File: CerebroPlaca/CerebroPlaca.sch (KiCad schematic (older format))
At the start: 39 parts

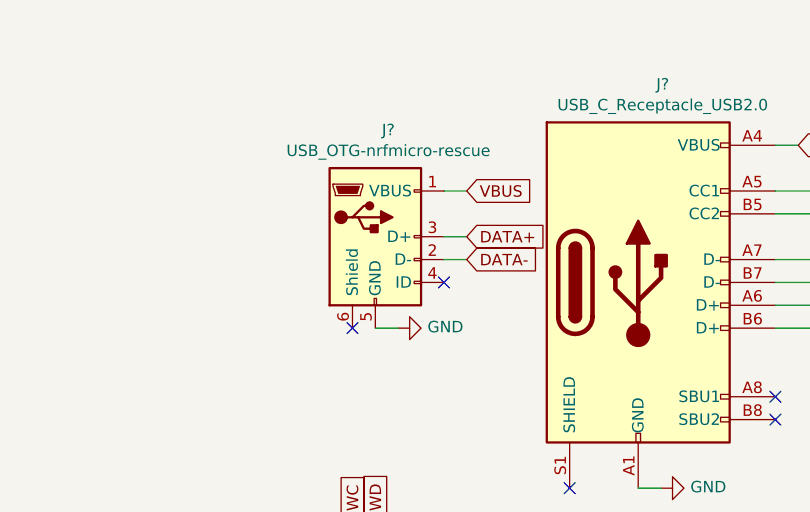
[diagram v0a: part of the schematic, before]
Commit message: se queda con el USB-C
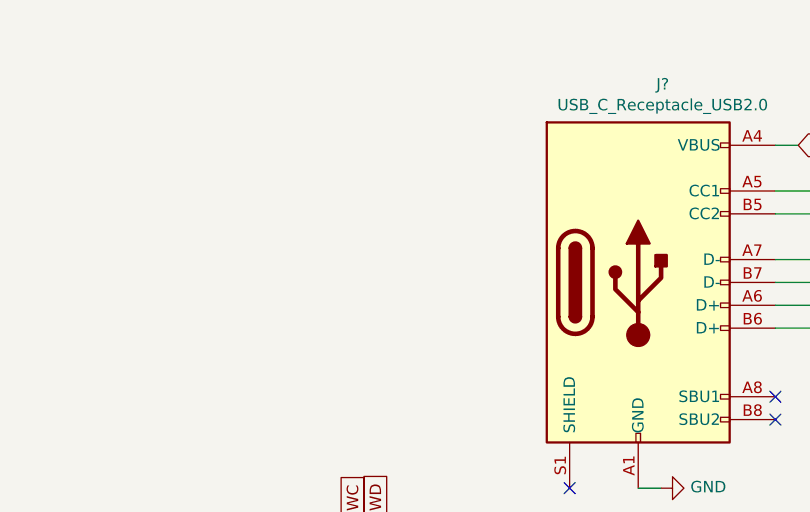
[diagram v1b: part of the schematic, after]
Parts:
- removed J?: USB_OTG-nrfmicro-rescue, symbol cerebro-rescue:USB_OTG-nrfmicro-rescue
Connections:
- no-connect marks 7 -> 5
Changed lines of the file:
@@
 P0.26
-$Comp
-L cerebro-rescue:USB_OTG-nrfmicro-rescue J?
-U 1 1 5E504B1F
-P 5400 1700
-F 0 "J?" H 5457 2167 50  0000 C CNN
-F 1 "USB_OTG-nrfmicro-rescue" H 5457 2076 50  0000 C CNN
-F 2 "" H 5550 1650 50  0001 C CNN
-F 3 "" H 5550 1650 50  0001 C CNN
-	1    5400 1700
-	1    0    0    -1
-$EndComp
 $Comp
 L Connector:USB_C_Receptacle_USB2.0 J?
@@
 	7900 1600 7800 1600
 Connection ~ 7900 1550
-NoConn ~ 5300 2100
-NoConn ~ 5700 1900
-$Comp
-L nrfmicro-rescue:GND #PWR0115
-U 1 1 5E52C5DE
-P 5500 2100
-F 0 "#PWR0115" H 5500 1850 50  0001 C CNN
-F 1 "GND" V 5505 1972 50  0000 R CNN
-F 2 "" H 5500 2100 50  0001 C CNN
-F 3 "" H 5500 2100 50  0001 C CNN
-	1    5500 2100
-	0    -1   -1   0
-$EndComp
-Wire Wire Line
-	5500 2100 5400 2100
-Text GLabel 5800 1800 2    50   Input ~ 0
-DATA-
-Text GLabel 5800 1700 2    50   Input ~ 0
-DATA+
-Wire Wire Line
-	5700 1700 5800 1700
-Wire Wire Line
-	5800 1800 5700 1800
-Text GLabel 5800 1500 2    50   Input ~ 0
-VBUS
-Wire Wire Line
-	5800 1500 5700 1500
 $Comp
 L cerebro-cache:Connector_Generic_Conn_01x02 J?
